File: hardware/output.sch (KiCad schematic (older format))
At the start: 94 parts, among them J79 Conn_01x03, J80 Conn_01x03, J81 Conn_01x03, J82 Screw_Terminal_01x04, J83 Conn_01x03, J84 Conn_01x03, J85 Conn_01x03, J86 Conn_01x03, J87 Conn_01x03, Q10 AO3400, Q12 AO3400, Q13 AO3400, Q3 AO3400, Q4 AO3400, Q5 AO3400, Q6 AON7418, Q7 AON7418, Q8 AO3400, Q9 AO3400, U7 IR4427S

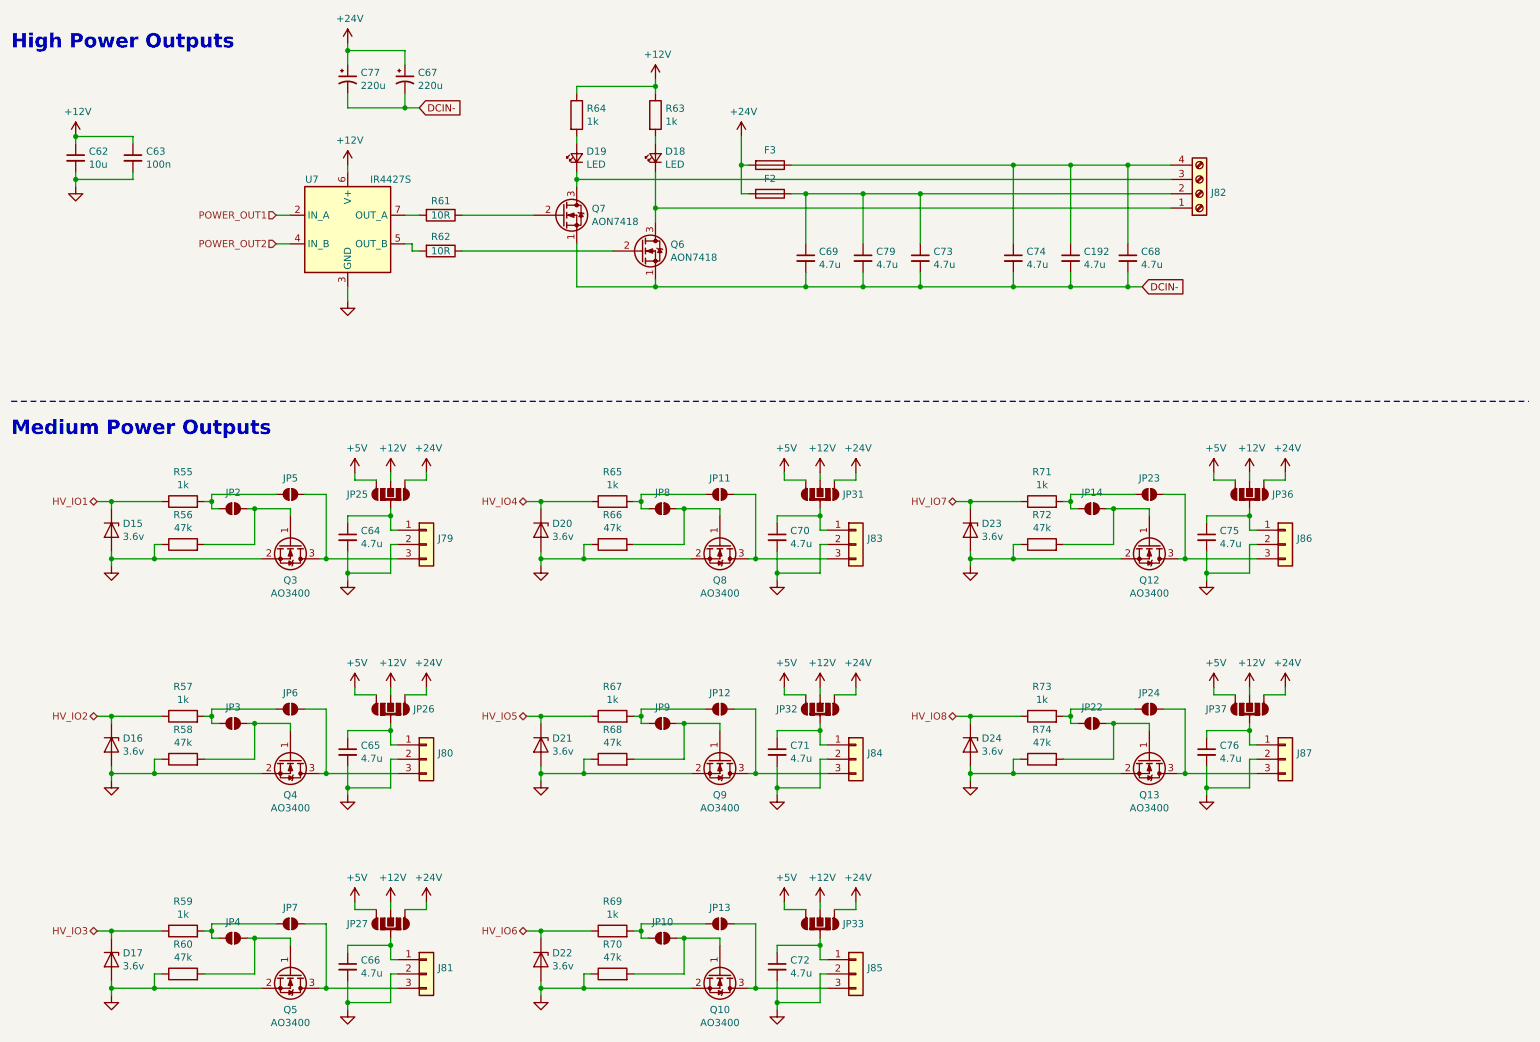
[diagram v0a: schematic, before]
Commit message: combine
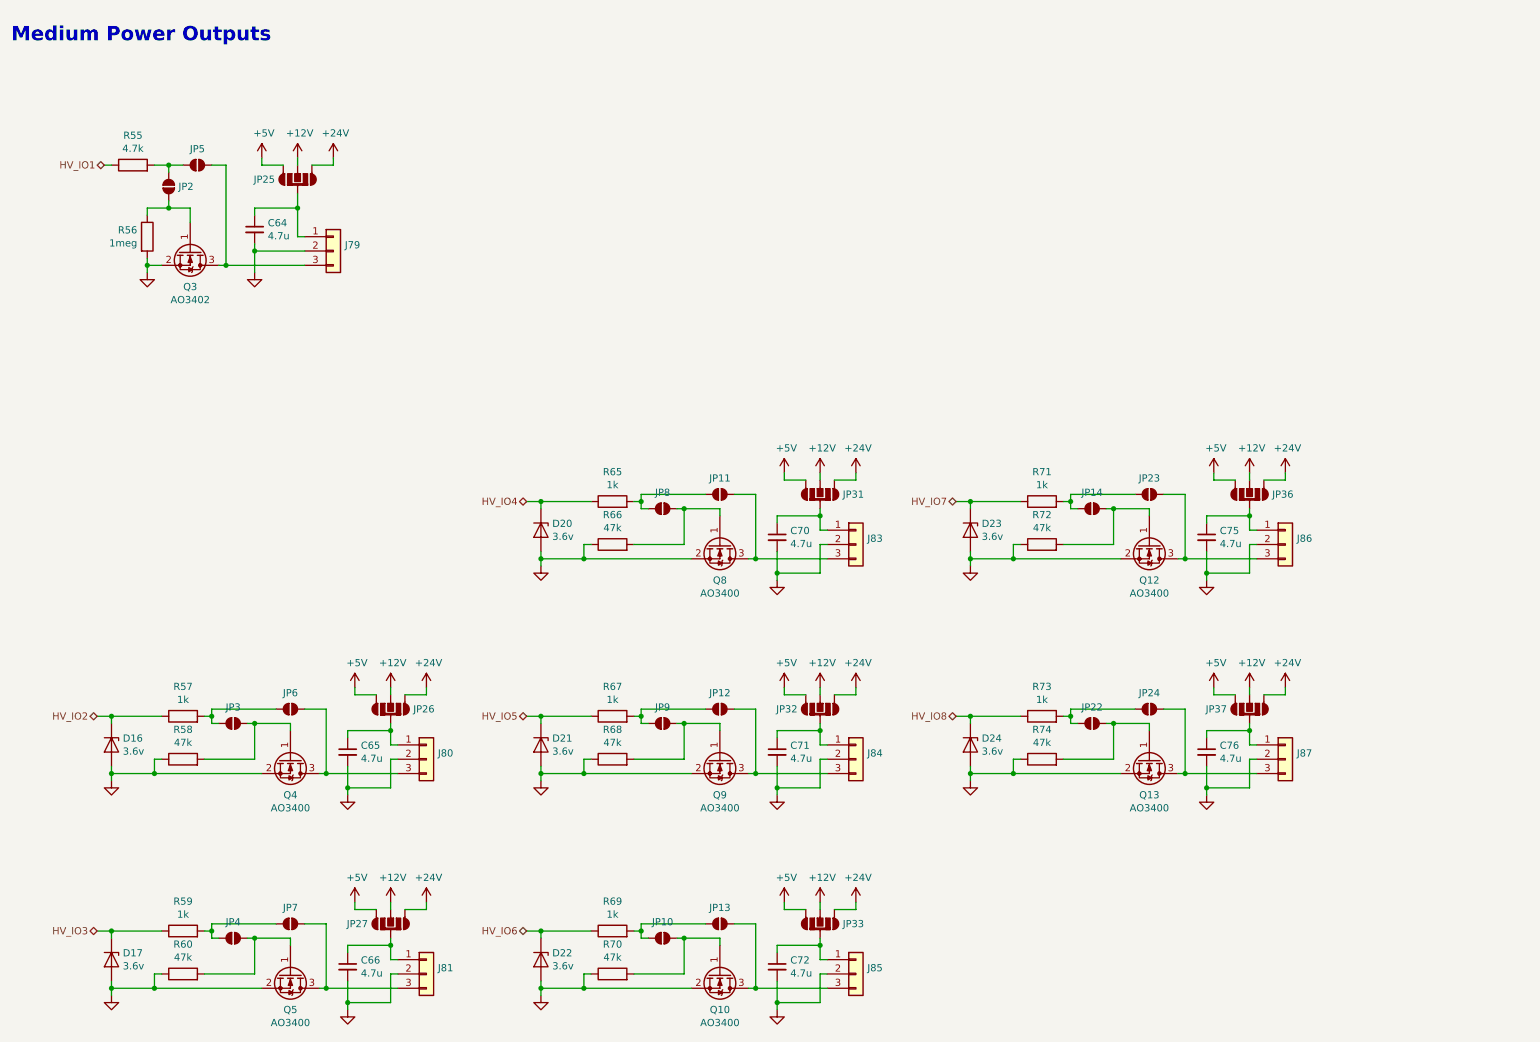
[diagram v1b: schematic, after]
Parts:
- removed C192, C68, C69, C73, C74, C79: 4.7u, _Generic:1210_CAP, symbol Device:C_Small
- removed C62: 10u, _Generic:0603_CAP, symbol Device:C_Small
- removed C63: 100n, _Generic:0603_CAP, symbol Device:C_Small
- removed C67, C77: 220u, Capacitor_SMD:CP_Elec_6.3x7.7, symbol Device:CP1_Small
- removed D15: 3.6v, _Generic:SOD-523_DIODE, symbol Device:D_Zener
- removed D18, D19: LED, _Generic:0603_LED, symbol Device:LED_Small
- removed F2, F3: Fuse, _Generic:1206_RES, symbol Device:Fuse
- removed J82: Screw_Terminal_01x04, _Generic:KF635-4P, symbol Connector:Screw_Terminal_01x04
- removed Q6, Q7: AON7418, _Generic:DFN3x3A_8L_EP1_P, symbol Device:Q_NMOS_SGD
- removed R61, R62: 10R, _Generic:0603_RES, symbol Device:R
- removed R63, R64: 1k, _Generic:0603_RES, symbol Device:R
- removed U7: IR4427S, _Generic:SO-8, symbol Driver_FET:MIC4427
- Q3: value AO3400 -> AO3402
- R55: value 1k -> 4.7k
- R56: value 47k -> 1meg
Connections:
- net GND: now also R56.2; no longer R56.1
- net at JP2.1 (A), R55.2: now also JP5.2 (B); no longer JP5.1 (A)
- net at J79.3 (Pin_3), Q3.3 (D): now also JP5.1 (A); no longer JP5.2 (B)
- net at JP2.2 (B), Q3.1 (G): now also R56.1; no longer R56.2
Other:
- note removed: "High Power Outputs"
- moved on the sheet: C64, J79, JP2, JP25, JP5, Q3, R55, R56

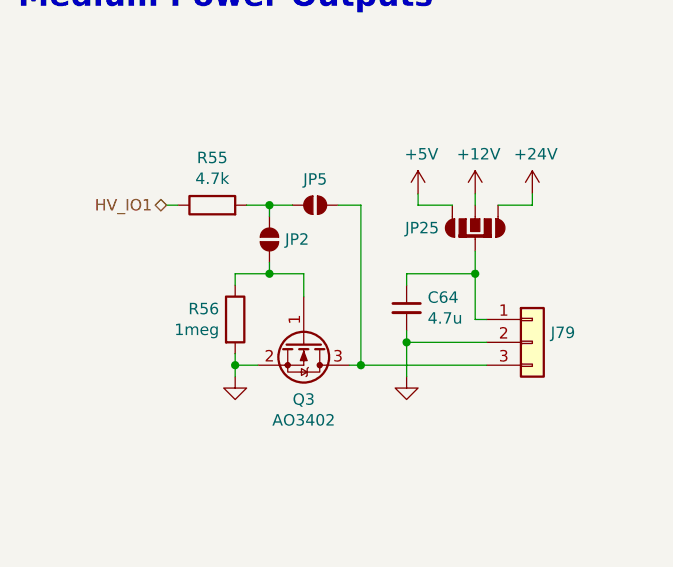
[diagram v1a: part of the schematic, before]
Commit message: new con
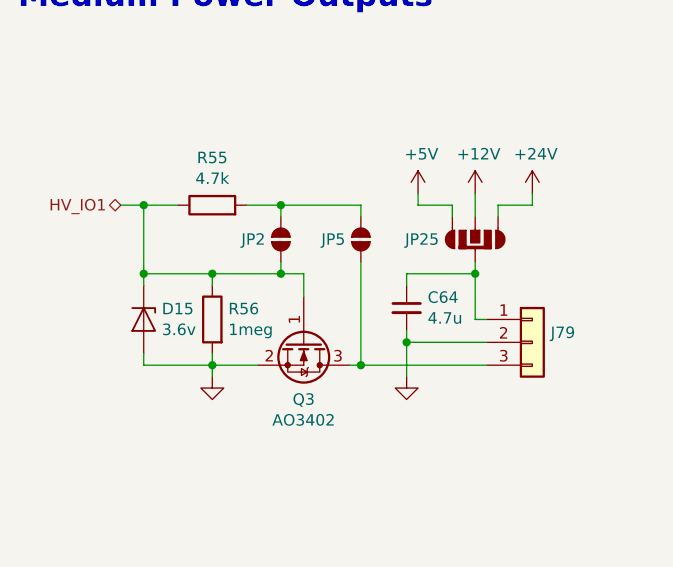
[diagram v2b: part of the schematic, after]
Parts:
- added D15: 3.6v, _Generic:SOD-523_DIODE, symbol Device:D_Zener
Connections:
- net GND: now also D15.2 (A)
- net HV_IO1: now also JP2.2 (B), Q3.1 (G), R56.1, D15.1 (K)
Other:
- moved on the sheet: JP2, JP25, JP5, R56
